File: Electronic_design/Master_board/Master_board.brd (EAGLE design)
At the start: 100 x 80 mm, 36 parts, among them IC1 74LS241N

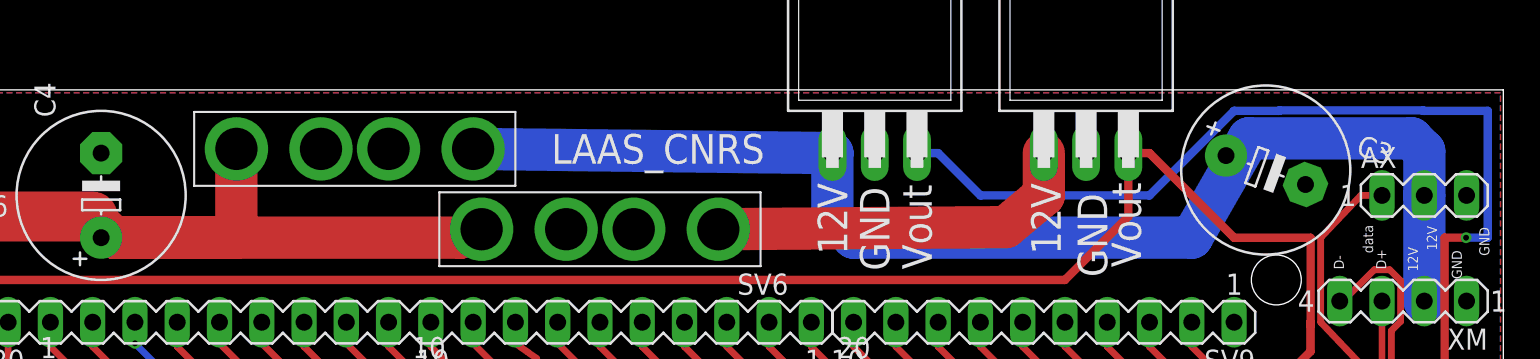
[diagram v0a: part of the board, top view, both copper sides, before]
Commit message: CRC OK
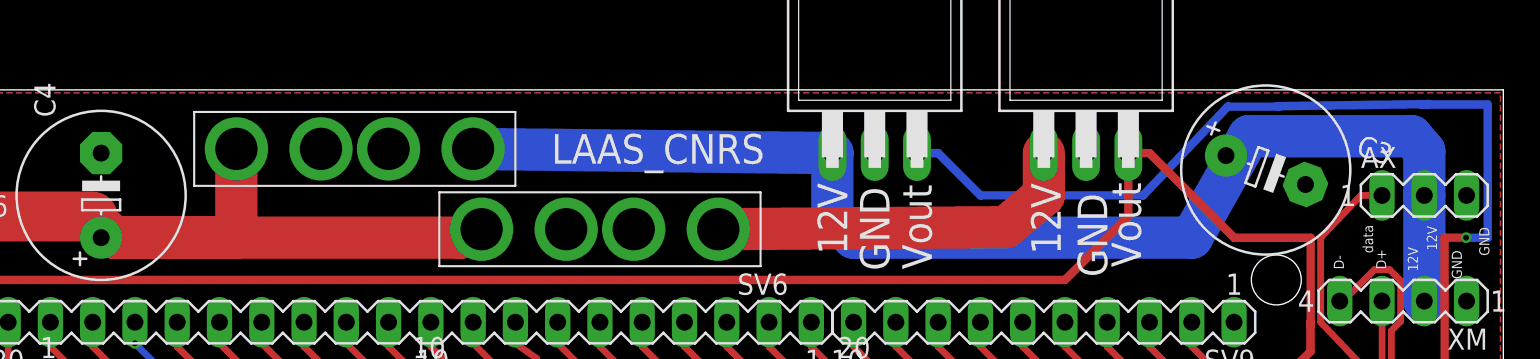
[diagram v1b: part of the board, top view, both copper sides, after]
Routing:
- net VCC: track 99.8 -> 101.5 mm
- net VIN: track 51.7 -> 52.5 mm
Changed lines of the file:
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@@
 <wire x1="64.77" y1="76.2" x2="66.04" y2="76.2" width="0.508" layer="16"/>
 <wire x1="66.04" y1="76.2" x2="68.58" y2="73.66" width="0.508" layer="16"/>
-<wire x1="68.58" y1="73.66" x2="78.74" y2="73.66" width="0.508" layer="16"/>
-<wire x1="83.82" y1="78.74" x2="86.52920625" y2="78.74" width="0.508" layer="16"/>
-<wire x1="86.52920625" y1="78.74" x2="86.55460625" y2="78.7654" width="0.508" layer="16"/>
-<wire x1="95.18239375" y1="78.7654" x2="95.20779375" y2="78.74" width="0.508" layer="16"/>
-<wire x1="95.20779375" y1="78.74" x2="99.06" y2="78.74" width="0.508" layer="16"/>
-<wire x1="86.55460625" y1="78.7654" x2="95.18239375" y2="78.7654" width="0.508" layer="16"/>
-<wire x1="99.06" y1="78.74" x2="99.06" y2="71.12" width="0.508" layer="16"/>
+<wire x1="68.58" y1="73.66" x2="78.359" y2="73.66" width="0.508" layer="16"/>
+<wire x1="83.439" y1="78.994" x2="86.52920625" y2="78.994" width="0.508" layer="16"/>
+<wire x1="86.52920625" y1="78.994" x2="86.42760625" y2="79.0194" width="0.508" layer="16"/>
+<wire x1="95.56339375" y1="79.1464" x2="95.08079375" y2="79.121" width="0.508" layer="16"/>
+<wire x1="95.08079375" y1="79.121" x2="99.06" y2="79.121" width="0.508" layer="16"/>
+<wire x1="86.42760625" y1="79.0194" x2="95.56339375" y2="79.1464" width="0.508" layer="16"/>
+<wire x1="99.06" y1="79.121" x2="99.06" y2="71.12" width="0.508" layer="16"/>
 <wire x1="99.06" y1="71.12" x2="97.7618" y2="71.12" width="0.508" layer="16"/>
 <via x="97.7618" y="71.12" extent="1-16" drill="0.35"/>
-<wire x1="78.74" y1="73.66" x2="83.82" y2="78.74" width="0.508" layer="16"/>
+<wire x1="78.359" y1="73.66" x2="83.439" y2="78.994" width="0.508" layer="16"/>
 <wire x1="97.7618" y1="71.12" x2="96.4726625" y2="71.12" width="0.508" layer="1"/>
 </signal>
@@
 <wire x1="59.69" y1="76.2" x2="59.69" y2="72.39" width="2.54" layer="16"/>
 <wire x1="59.69" y1="72.39" x2="60.96" y2="71.12" width="2.54" layer="16"/>
-<wire x1="84.709" y1="77.089" x2="94.488" y2="77.089" width="2.54" layer="16"/>
-<wire x1="94.488" y1="77.089" x2="95.25" y2="76.327" width="2.54" layer="16"/>
+<wire x1="84.709" y1="77.216" x2="94.488" y2="77.216" width="2.54" layer="16"/>
+<wire x1="94.488" y1="77.216" x2="95.25" y2="76.327" width="2.54" layer="16"/>
 <wire x1="95.25" y1="76.327" x2="95.25" y2="73.66" width="2.54" layer="16"/>
 <wire x1="81.28" y1="71.12" x2="60.96" y2="71.12" width="2.54" layer="16"/>
-<wire x1="81.28" y1="71.12" x2="84.709" y2="77.089" width="2.54" layer="16"/>
+<wire x1="81.28" y1="71.12" x2="84.709" y2="77.216" width="2.54" layer="16"/>
 <wire x1="95.25" y1="73.66" x2="95.25" y2="67.31" width="2.54" layer="16"/>
 <contactref element="C3" pad="+"/>
@@
 <wire x1="15.24" y1="72.39" x2="16.51" y2="71.12" width="2.54" layer="1"/>
 <contactref element="C4" pad="+"/>
-<wire x1="16.51" y1="71.12" x2="15.748" y2="71.12" width="0" layer="19" extent="1-1"/>
+<wire x1="15.748" y1="71.12" x2="16.51" y2="71.12" width="0.1524" layer="1"/>
 </signal>
 <signal name="3V3">
